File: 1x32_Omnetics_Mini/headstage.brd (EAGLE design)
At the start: 100 x 80 mm, 13 parts, among them U1 RHD2132_QFN

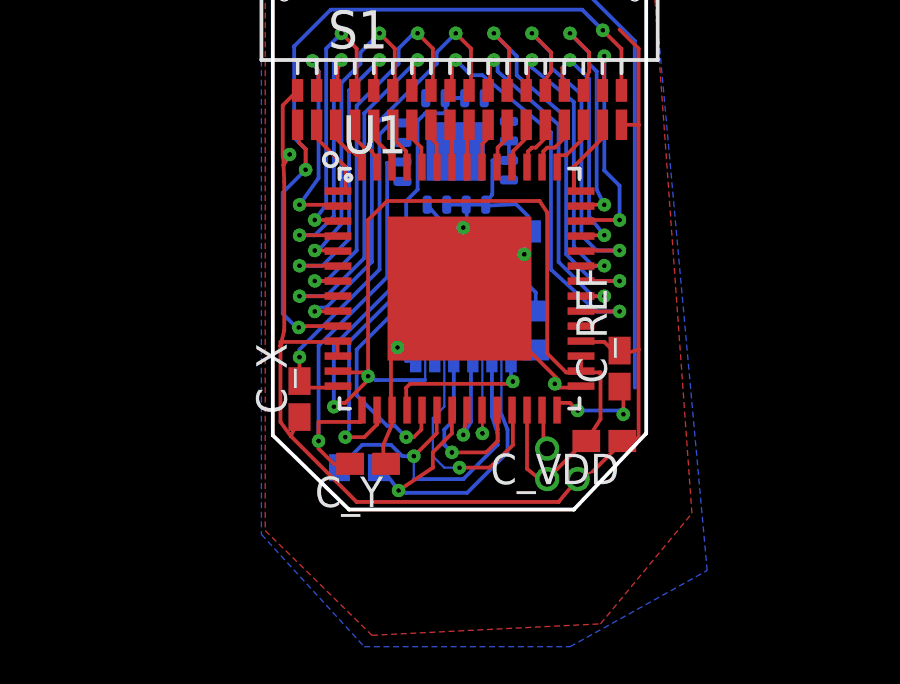
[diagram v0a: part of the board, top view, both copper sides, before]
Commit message: Cosmetic cleanups
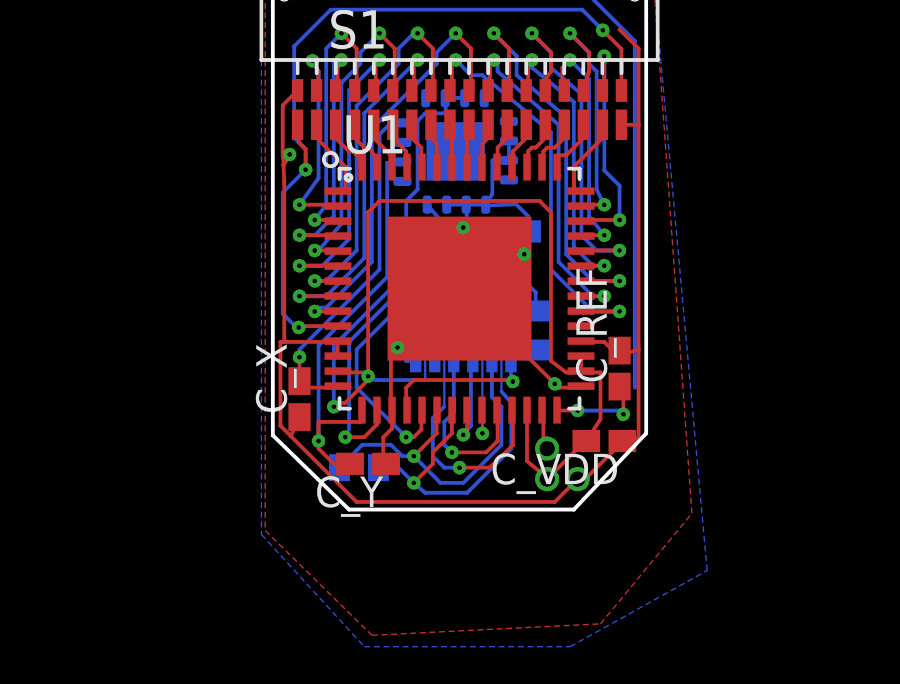
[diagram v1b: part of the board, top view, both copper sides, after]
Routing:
- net SCLK+: track 13.9 -> 13.3 mm
